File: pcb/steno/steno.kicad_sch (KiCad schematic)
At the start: 63 parts, among them J1 Conn_01x04, K1 diode-choc, K10 diode-choc, K11 diode-choc, K12 diode-choc, K13 diode-choc, K14 diode-choc, K15 diode-choc, K16 diode-choc, K17 diode-choc, K18 diode-choc, K19 diode-choc, K2 diode-choc, K20 diode-choc, K21 diode-choc, K22 diode-choc, K23 diode-choc, K24 diode-choc, K25 diode-choc, K26 diode-choc, K27 diode-choc, K28 diode-choc, K29 diode-choc, K3 diode-choc, K30 diode-choc, K31 diode-choc, K32 diode-choc, K33 diode-choc, K34 diode-choc, K35 diode-choc, K36 diode-choc, K37 diode-choc, K38 diode-choc, K39 diode-choc, K4 diode-choc, K40 diode-choc, K5 diode-choc, K6 diode-choc, K7 diode-choc, K8 diode-choc, K9 diode-choc, Q1 AO3401A, SW2 SW_Push, U1 MT25QL128ABA1ESE, U2 holyiot-18010-no-underside

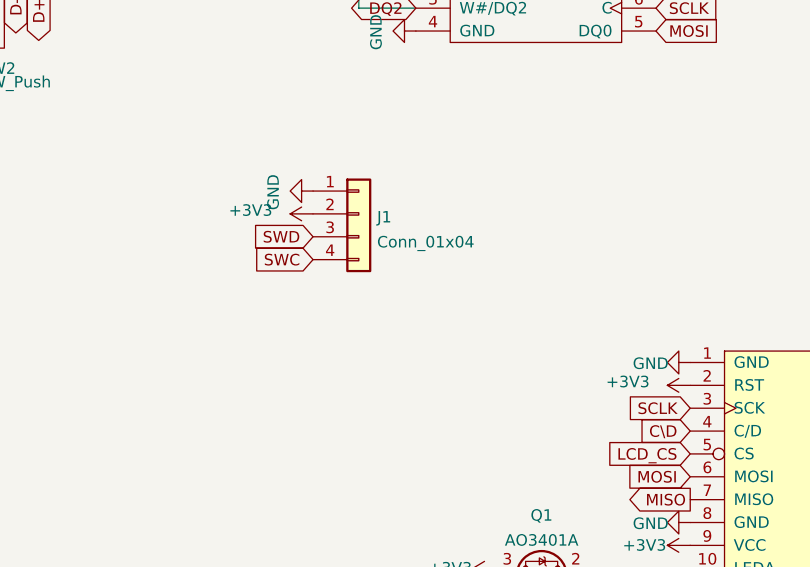
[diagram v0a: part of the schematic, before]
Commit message: [pcb] Auklet 3: first revision
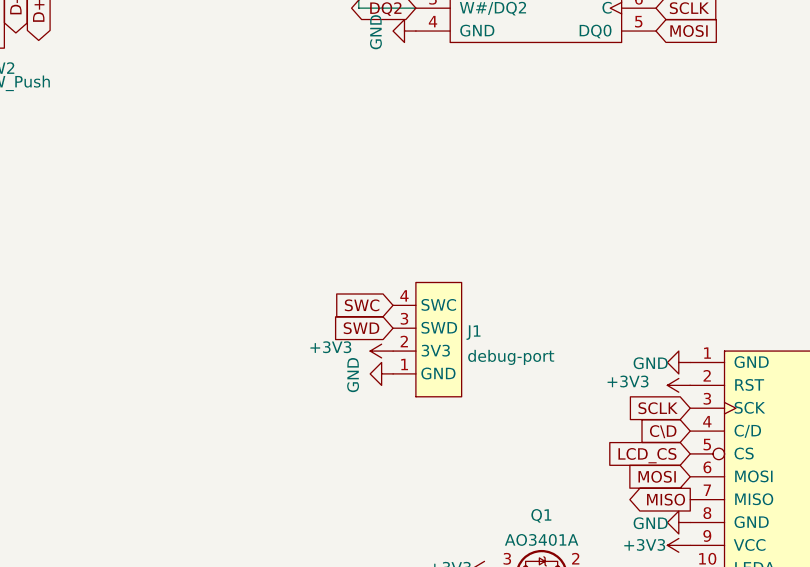
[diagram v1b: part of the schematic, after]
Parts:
- removed J1: Conn_01x04, keeb-libs:debug-port-single-side, symbol Connector_Generic:Conn_01x04
- added J1: debug-port, misc:debug-port-single-side, symbol misc:debug-port
- U2: footprint mcu:Holyiot-18010-no-underside -> mcu:holyiot-18010-no-underside
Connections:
- net +3V3: now also J1.2 (3V3)
- net GND: now also J1.1 (GND)
- net SWC: now also J1.4 (SWC)
- net SWD: now also J1.3 (SWD)
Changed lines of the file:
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@@
     )
   )
-  (global_label "SWD" (shape input) (at 119.38 110.49 180) (fields_autoplaced)
-    (effects (font (size 1.27 1.27)) (justify right))
-    (property "Intersheet References" "${INTERSHEET_REFS}" (id 0) (at 113.0359 110.4106 0)
-      (effects (font (size 1.27 1.27)) (justify right) hide)
-    )
-  )
-  (global_label "SWC" (shape input) (at 119.38 113.03 180) (fields_autoplaced)
-    (effects (font (size 1.27 1.27)) (justify right))
-    (property "Intersheet References" "${INTERSHEET_REFS}" (id 0) (at 113.0359 112.9506 0)
+  (global_label "SWD" (shape input) (at 128.27 120.65 180) (fields_autoplaced)
+    (effects (font (size 1.27 1.27)) (justify right))
+    (property "Intersheet References" "${INTERSHEET_REFS}" (id 0) (at 121.9259 120.5706 0)
+      (effects (font (size 1.27 1.27)) (justify right) hide)
+    )
+  )
+  (global_label "SWC" (shape input) (at 128.27 118.11 180) (fields_autoplaced)
+    (effects (font (size 1.27 1.27)) (justify right))
+    (property "Intersheet References" "${INTERSHEET_REFS}" (id 0) (at 121.9259 118.0306 0)
       (effects (font (size 1.27 1.27)) (justify right) hide)
     )
@@
     (pin "2")
   )
-  (symbol (lib_id "power:+3V3") (at 119.38 107.95 90) (unit 1)
-    (in_bom yes) (on_board yes)
-    (property "Reference" "#PWR06" (id 0) (at 123.19 107.95 0)
-      (effects (font (size 1.27 1.27)) hide)
-    )
-    (property "Value" "+3V3" (id 1) (at 112.4458 107.569 90))
-    (property "Footprint" "" (id 2) (at 119.38 107.95 0)
-      (effects (font (size 1.27 1.27)) hide)
-    )
-    (property "Datasheet" "" (id 3) (at 119.38 107.95 0)
+  (symbol (lib_id "power:+3V3") (at 128.27 123.19 90) (unit 1)
+    (in_bom yes) (on_board yes)
+    (property "Reference" "#PWR06" (id 0) (at 132.08 123.19 0)
+      (effects (font (size 1.27 1.27)) hide)
+    )
+    (property "Value" "+3V3" (id 1) (at 121.3358 122.809 90))
+    (property "Footprint" "" (id 2) (at 128.27 123.19 0)
+      (effects (font (size 1.27 1.27)) hide)
+    )
+    (property "Datasheet" "" (id 3) (at 128.27 123.19 0)
       (effects (font (size 1.27 1.27)) hide)
     )
@@
     (property "Reference" "U2" (id 0) (at 76.2 27.9105 0))
     (property "Value" "holyiot-18010-no-underside" (id 1) (at 76.2 30.6856 0))
-    (property "Footprint" "mcu:Holyiot-18010-no-underside" (id 2) (at 114.3 73.66 0)
+    (property "Footprint" "mcu:holyiot-18010-no-underside" (id 2) (at 114.3 73.66 0)
       (effects (font (size 1.27 1.27)) hide)
     )
@@
     (pin "2")
   )
-  (symbol (lib_id "power:GND") (at 119.38 105.41 270) (unit 1)
-    (in_bom yes) (on_board yes)
-    (property "Reference" "#PWR05" (id 0) (at 113.03 105.41 0)
-      (effects (font (size 1.27 1.27)) hide)
-    )
-    (property "Value" "GND" (id 1) (at 114.9858 105.537 0))
-    (property "Footprint" "" (id 2) (at 119.38 105.41 0)
-      (effects (font (size 1.27 1.27)) hide)
-    )
-    (property "Datasheet" "" (id 3) (at 119.38 105.41 0)
+  (symbol (lib_id "misc:debug-port") (at 132.08 121.92 90) (unit 1)
+    (in_bom no) (on_board yes) (fields_autoplaced)
+    (property "Reference" "J1" (id 0) (at 136.525 121.0115 90)
+      (effects (font (size 1.27 1.27)) (justify right))
+    )
+    (property "Value" "debug-port" (id 1) (at 136.525 123.7866 90)
+      (effects (font (size 1.27 1.27)) (justify right))
+    )
+    (property "Footprint" "misc:debug-port-single-side" (id 2) (at 139.7 121.92 0)
+      (effects (font (size 1.27 1.27)) hide)
+    )
+    (property "Datasheet" "" (id 3) (at 132.08 121.92 0)
+      (effects (font (size 1.27 1.27)) hide)
+    )
+    (pin "1")
+    (pin "2")
+    (pin "3")
+    (pin "4")
+  )
+  (symbol (lib_id "power:GND") (at 128.27 125.73 270) (unit 1)
+    (in_bom yes) (on_board yes)
+    (property "Reference" "#PWR05" (id 0) (at 121.92 125.73 0)
+      (effects (font (size 1.27 1.27)) hide)
+    )
+    (property "Value" "GND" (id 1) (at 123.8758 125.857 0))
+    (property "Footprint" "" (id 2) (at 128.27 125.73 0)
+      (effects (font (size 1.27 1.27)) hide)
+    )
+    (property "Datasheet" "" (id 3) (at 128.27 125.73 0)
       (effects (font (size 1.27 1.27)) hide)
     )
@@
     (pin "1")
     (pin "2")
-  )
-  (symbol (lib_id "Connector_Generic:Conn_01x04") (at 124.46 107.95 0) (unit 1)
-    (in_bom yes) (on_board yes) (fields_autoplaced)
-    (property "Reference" "J1" (id 0) (at 126.4921 108.3115 0)
-      (effects (font (size 1.27 1.27)) (justify left))
-    )
-    (property "Value" "Conn_01x04" (id 1) (at 126.4921 111.0866 0)
-      (effects (font (size 1.27 1.27)) (justify left))
-    )
-    (property "Footprint" "keeb-libs:debug-port-single-side" (id 2) (at 124.46 107.95 0)
-      (effects (font (size 1.27 1.27)) hide)
-    )
-    (property "Datasheet" "~" (id 3) (at 124.46 107.95 0)
-      (effects (font (size 1.27 1.27)) hide)
-    )
-    (pin "1")
-    (pin "2")
-    (pin "3")
-    (pin "4")
   )
   (symbol (lib_id "Device:Battery_Cell") (at 35.56 73.66 90) (unit 1)
@@
       (reference "H2") (unit 1) (value "MountingHole") (footprint "misc:auklet-cover-mount")
     )
-    (path "/847ba160-b305-4501-94eb-1e40ac133731"
-      (reference "J1") (unit 1) (value "Conn_01x04") (footprint "keeb-libs:debug-port-single-side")
+    (path "/51f1c228-b893-4ab5-bdfa-2eae1932a96d"
+      (reference "J1") (unit 1) (value "debug-port") (footprint "misc:debug-port-single-side")
     )
     (path "/144bad29-9f29-444f-a7e7-dc1674e796e3/9cfa9adb-81c6-4c01-b5f5-5a8080a68a7c"
@@
     )
     (path "/2086f1f4-059c-4ac4-858b-c6e65c5b1092"
-      (reference "U2") (unit 1) (value "holyiot-18010-no-underside") (footprint "mcu:Holyiot-18010-no-underside")
+      (reference "U2") (unit 1) (value "holyiot-18010-no-underside") (footprint "mcu:holyiot-18010-no-underside")
     )
     (path "/144bad29-9f29-444f-a7e7-dc1674e796e3/70f4f660-4e28-4704-85fb-b723fc879f87"
